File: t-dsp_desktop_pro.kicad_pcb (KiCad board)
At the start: 8 copper layers, 120 x 100 mm, 155 parts, among them IC1 Logic Level Shifter - 74HCT2G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, J1 jumper, J10 JST-XH Connector, J11 JST-XH Connector, J12 RGB LED HEADEER, J13 Conn_01x02, J15 Conn_01x01, J16 Conn_01x02, J17 Conn_02x04_Odd_Even, J18 Conn_02x02_Odd_Even, J19 Conn_01x01, J2 GROUND HEADER, J20 Conn_01x01, J21 jumper, J3 jumper, J4 jumper, J5 jumper, J6 jumper, J7 jumper, J8 PJRAS2X1S01X, J9 PJRAS2X1S01X, Q1 DMG2307L-7, Q2 DMG2307L-7, T108 Tab, T109 Tab, T110 Tab, T111 Tab, U1 Teensy 4.1 - DEVKIT, U10 TPD4E02B04DQA, U2 ESP32-DevKitC - DEVKIT, U3 Power Mux & Protect - TPS2116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, U4 Optoisolators - H11L1SM - 6-S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, U5 Dual Buffer - SN74LVC2G125DCTR, U6 Dual Buffer - SN74LVC2G125DCTR, U7 Dual Buffer - SN74LVC2G125DCTR, U8 Dual Buffer - SN74LVC2G125DCTR, U9 Dual Buffer - 74HCT2G17GW,125

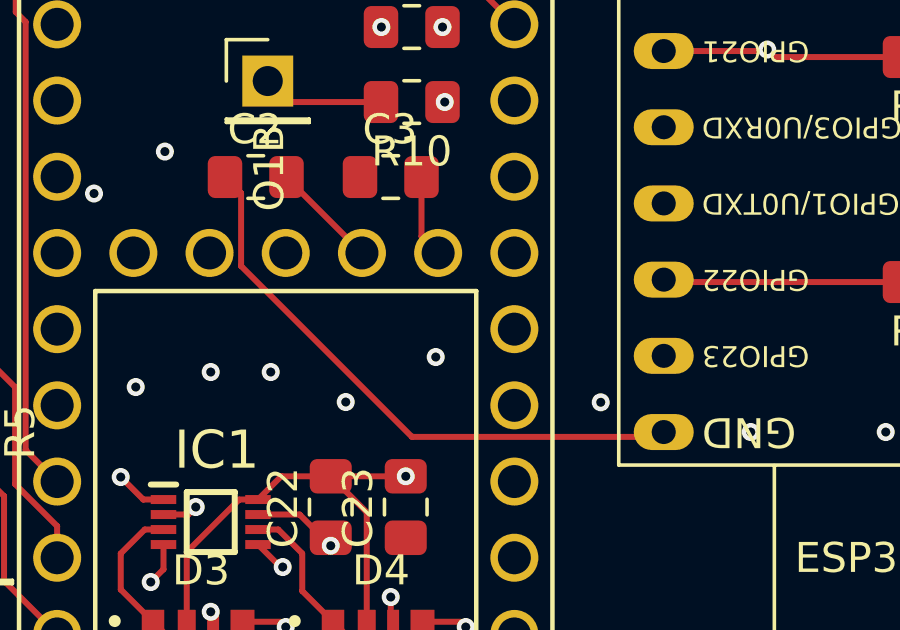
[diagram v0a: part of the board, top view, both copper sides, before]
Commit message: v0.8.4: Production release - final layout and schematic updates
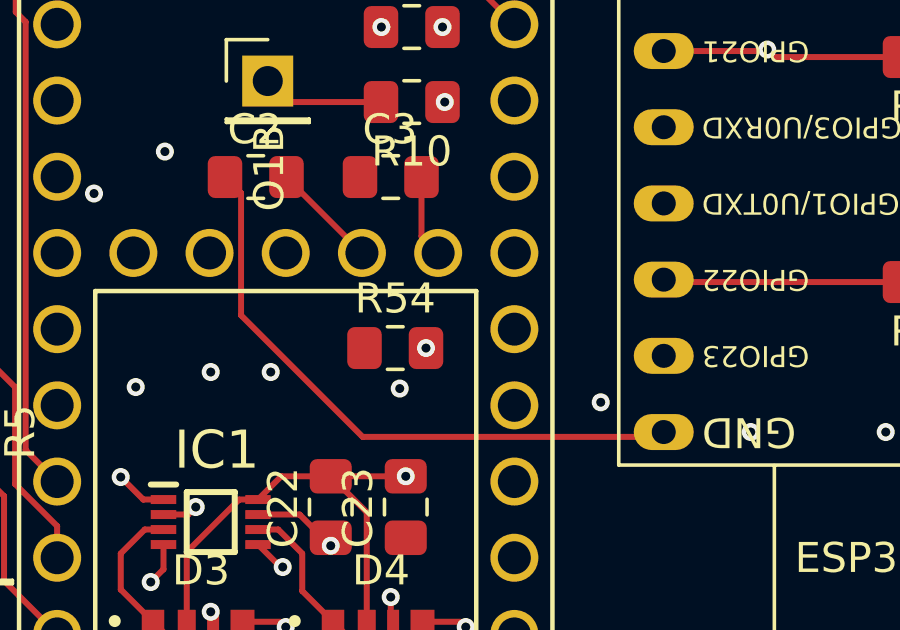
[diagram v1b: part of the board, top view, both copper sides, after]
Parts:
- added R54: 10k, project_fp:R_0805_2012Metric_Pad1.15x1.40mm_HandSolder, F.Cu at (171.7, 189.2)
- R11: value 2.21k ohm -> 10k
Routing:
- net 34_RX8_RESET2: track 160.7 -> 168.9 mm, vias 3 -> 4
- net HOST_D1-: track 51.7 -> 49.0 mm
- net GND: track 733.1 -> 734.1 mm, vias 330 -> 329
